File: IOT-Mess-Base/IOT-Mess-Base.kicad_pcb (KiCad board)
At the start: 2 copper layers, 24.1 x 24.5 mm, 30 parts, among them J1 Conn_01x09_Pin, J2 TP_4056, Q1 AO3400A, Q2 AO3401A, Q3 AO3400A, Q4 AO3401A, Q5 AO3400A, SW2 SW_Push, SW3 SW_Push, U12 APDS-9960, U13 SHT31-DIS, U17 BH1750FVI-TR, U2 SHT4x, U3 INA219AxDCN, U8 TPL5110

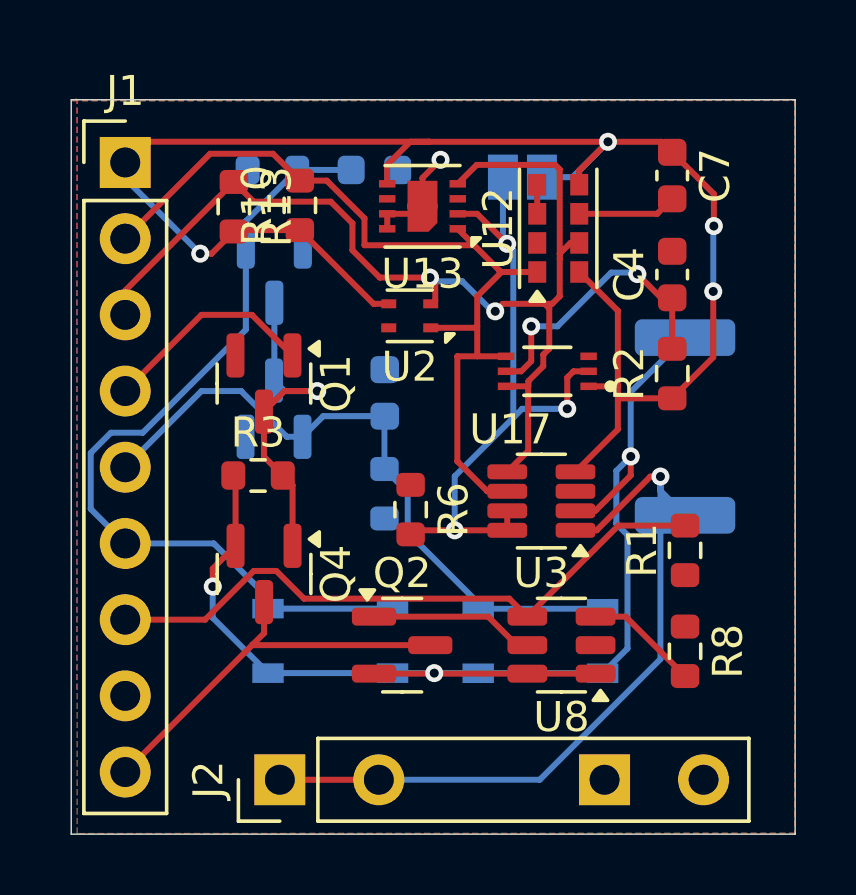
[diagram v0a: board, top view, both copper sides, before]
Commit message: did some works.
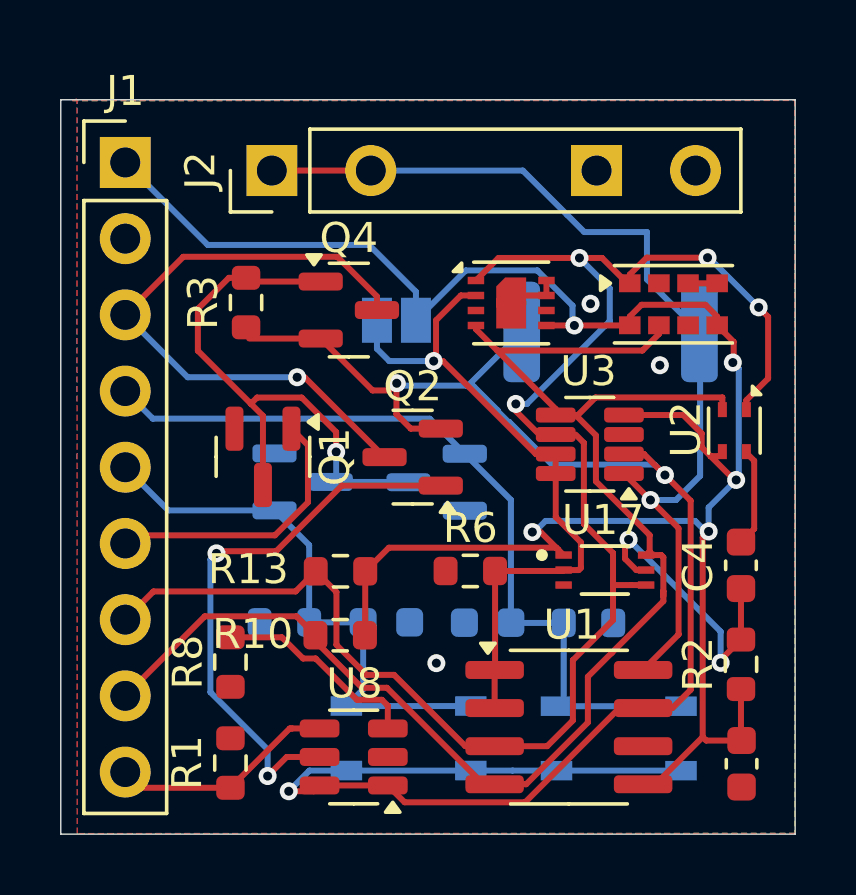
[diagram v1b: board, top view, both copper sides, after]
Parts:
- added U1: INA219AxD, Package_SO:SOIC-8_3.9x4.9mm_P1.27mm, F.Cu at (95.7, 91.5)
- moved J2 20.3 mm to (85.8, 73.0)
- moved C7 19.7 mm to (101.4, 92.7)
- moved R1 16.7 mm to (84.4, 92.7), turned to -90 degrees
- moved R8 15.2 mm to (84.4, 89.3), turned to 90 degrees
- moved C5 15.1 mm to (89.6, 88.0)
- moved R5 15.1 mm to (86.2, 88.0)
- moved R13 14.7 mm to (88.1, 88.4), turned to 0 degrees
- moved R10 12.3 mm to (88.1, 86.3), turned to 180 degrees
- moved U2 11.5 mm to (101.2, 81.6), turned to -90 degrees
- moved R2 9.96 mm to (101.4, 89.4)
- moved C4 9.96 mm to (101.4, 86.1)
- moved Q4 9.24 mm to (88.4, 77.6), turned to 0 degrees
- moved C6 8.39 mm to (93.0, 88.0), turned to 180 degrees
- moved R18 8.05 mm to (96.3, 88.0), turned to 180 degrees
- moved U8 7.86 mm to (88.5, 92.5)
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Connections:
- J1 pad 2: SDA_0 -> GND
- J1 pad 3: SCL_0 -> VCC
- J1 pad 4: DRIVE -> LSW0
- J1 pad 5: LSW0 -> LSW1
- J1 pad 6: LSW1 -> DRIVE
- J1 pad 7: DONE -> SDA_0
- J1 pad 8: GND -> SCL_0
- J1 pad 9: VCC -> DONE
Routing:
- net SDA_0: track 31.2 -> 55.1 mm, vias 0 -> 4
- net V-: track 41.8 -> 58.4 mm
- net DONE: track 21.2 -> 7.51 mm
- net SCL_0: track 36.3 -> 49.9 mm, vias 2 -> 0
- net Net-(Q2-G): track 5.15 -> 18.7 mm, vias 0 -> 2
- net +3.3V: track 57.3 -> 68.2 mm, vias 4 -> 5
- net LSW1: track 27.9 -> 18.8 mm
- net Net-(Q1-D): track 11.1 -> 19.2 mm
- net VCC: track 13.5 -> 20.8 mm, vias 0 -> 1
- net Vi+: track 25.6 -> 31.4 mm
- net LSW0: track 22.8 -> 27.4 mm
- net LR0: track 3.80 -> 6.95 mm
- net DRIVE: track 7.18 -> 9.34 mm
- net GND: track 6.89 -> 5.08 mm, vias 1 -> 3
- net ADDR: track 22.5 -> 23.0 mm, vias 3 -> 1
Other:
- board size 24.1 x 24.5 mm -> 24.5 x 24.5 mm
- board text added: "3.3"
- board text added: "B+"
- board text added: "B-"
- board text added: "DONE"
- board text added: "DRV"
- board text added: "GND"
- board text added: "IOT-Mess SENS V1.0"
- board text added: "SCL"
- board text added: "SDA"
- board text added: "SW0"
- board text added: "SW1"
- board text added: "VCC"
